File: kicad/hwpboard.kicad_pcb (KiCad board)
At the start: 2 copper layers, 100 x 80 mm, 5 parts, among them J1 Barrel_Jack_Switch, J2 Conn_01x01, J3 Conn_01x01, J4 Conn_01x01, J5 Conn_01x01

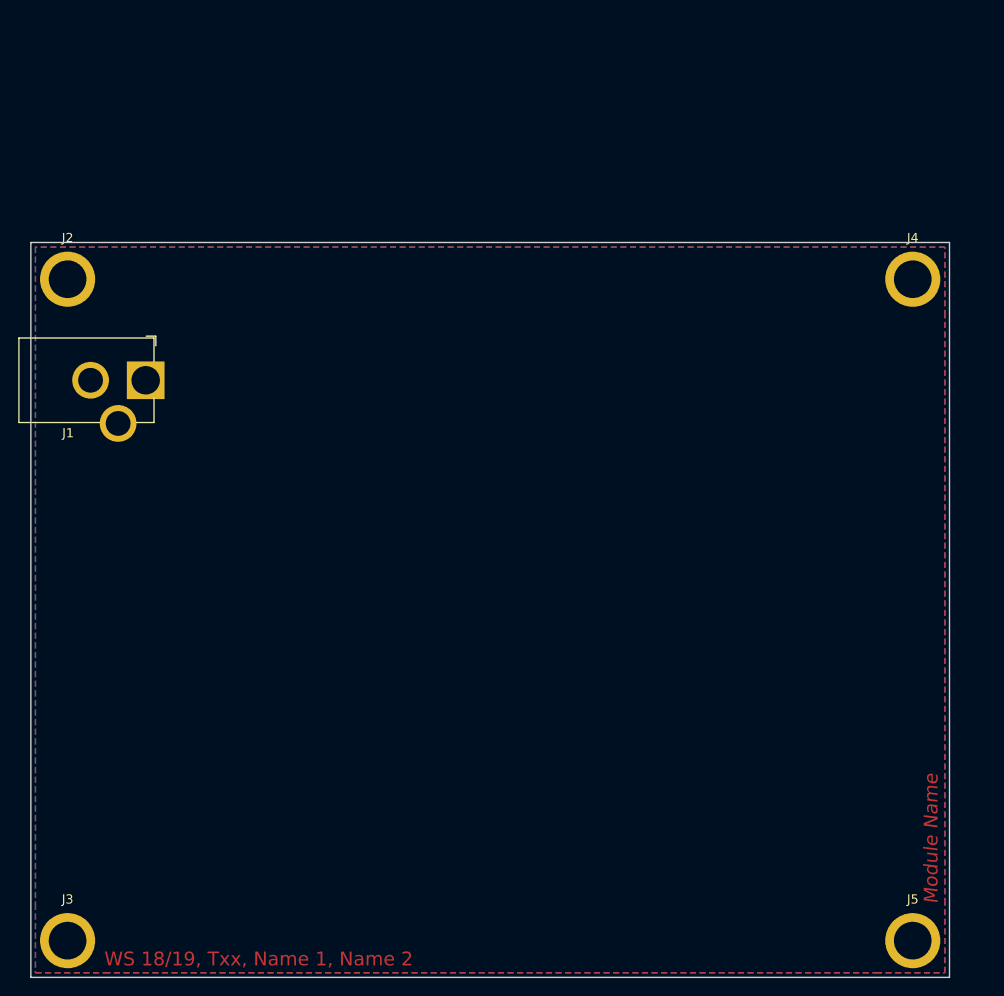
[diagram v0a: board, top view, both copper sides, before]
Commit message: schematic v1.0 ready
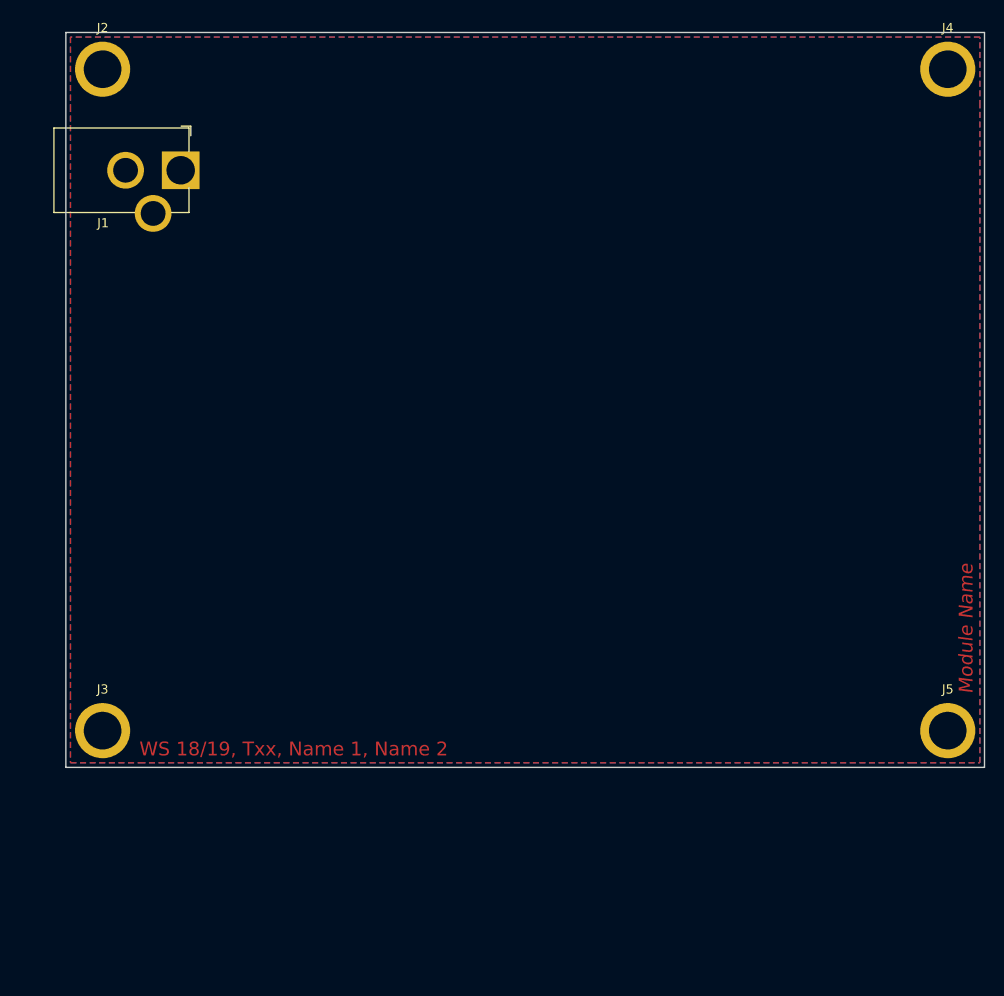
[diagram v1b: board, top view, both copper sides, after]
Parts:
- moved J1 23.2 mm to (121.3, 57.1)
- moved J2 23.2 mm to (112.8, 46.1)
- moved J3 23.2 mm to (112.8, 118.1)
- moved J4 23.2 mm to (204.8, 46.1)
- moved J5 23.2 mm to (204.8, 118.1)
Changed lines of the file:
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@@
-(kicad_pcb (version 20171130) (host pcbnew 5.0.0+dfsg1-2~bpo9+1)
+(kicad_pcb (version 20171130) (host pcbnew 5.0.0-fee4fd1~66~ubuntu18.04.1)
   (general
     (thickness 1.6)
@@
   )
   (module HWP:BarrelJack_Horizontal_CustomHWP (layer F.Cu)
-    (at 117.5 80)
+    (at 121.31 57.14)
     (descr "DC Barrel Jack")
     (tags "Power Jack")
@@
   )
   (module HWP:MountingHole_4.1mm_M4_ISO14580_Pad (layer F.Cu)
-    (at 109 69)
+    (at 112.81 46.14)
     (descr "Mounting Hole 4.3mm, M4, ISO14580")
     (tags "mounting hole 4.3mm m4 iso14580")
@@
   )
   (module HWP:MountingHole_4.1mm_M4_ISO14580_Pad (layer F.Cu)
-    (at 109 141)
+    (at 112.81 118.14)
     (descr "Mounting Hole 4.3mm, M4, ISO14580")
     (tags "mounting hole 4.3mm m4 iso14580")
@@
   )
   (module HWP:MountingHole_4.1mm_M4_ISO14580_Pad (layer F.Cu)
-    (at 201 69)
+    (at 204.81 46.14)
     (descr "Mounting Hole 4.3mm, M4, ISO14580")
     (tags "mounting hole 4.3mm m4 iso14580")
@@
   )
   (module HWP:MountingHole_4.1mm_M4_ISO14580_Pad (layer F.Cu)
-    (at 201 141)
+    (at 204.81 118.14)
     (descr "Mounting Hole 4.3mm, M4, ISO14580")
     (tags "mounting hole 4.3mm m4 iso14580")
@@
   )
   (dimension 80 (width 0.3) (layer Dwgs.User)
-    (gr_text "80 mm" (at 92.900001 105 270) (layer Dwgs.User)
+    (gr_text "80 mm" (at 118.300001 98.65 270) (layer Dwgs.User)
       (effects (font (size 1.5 1.5) (thickness 0.3)))
     )
-    (feature1 (pts (xy 100 145) (xy 94.41358 145)))
-    (feature2 (pts (xy 100 65) (xy 94.41358 65)))
-    (crossbar (pts (xy 95.000001 65) (xy 95.000001 145)))
-    (arrow1a (pts (xy 95.000001 145) (xy 94.41358 143.873496)))
-    (arrow1b (pts (xy 95.000001 145) (xy 95.586422 143.873496)))
-    (arrow2a (pts (xy 95.000001 65) (xy 94.41358 66.126504)))
-    (arrow2b (pts (xy 95.000001 65) (xy 95.586422 66.126504)))
-  )
-  (gr_text "Module Name" (at 203 137 90) (layer F.Cu)
+    (feature1 (pts (xy 125.4 138.65) (xy 119.81358 138.65)))
+    (feature2 (pts (xy 125.4 58.65) (xy 119.81358 58.65)))
+    (crossbar (pts (xy 120.400001 58.65) (xy 120.400001 138.65)))
+    (arrow1a (pts (xy 120.400001 138.65) (xy 119.81358 137.523496)))
+    (arrow1b (pts (xy 120.400001 138.65) (xy 120.986422 137.523496)))
+    (arrow2a (pts (xy 120.400001 58.65) (xy 119.81358 59.776504)))
+    (arrow2b (pts (xy 120.400001 58.65) (xy 120.986422 59.776504)))
+  )
+  (gr_text "Module Name" (at 206.81 114.14 90) (layer F.Cu)
     (effects (font (size 1.5 1.5) (thickness 0.2) italic) (justify left))
   )
-  (gr_text "WS 18/19, Txx, Name 1, Name 2" (at 113 143) (layer F.Cu)
+  (gr_text "WS 18/19, Txx, Name 1, Name 2" (at 116.81 120.14) (layer F.Cu)
     (effects (font (size 1.5 1.5) (thickness 0.2)) (justify left))
   )
   (dimension 100 (width 0.3) (layer Dwgs.User)
-    (gr_text "100 mm" (at 155 52.9) (layer Dwgs.User)
+    (gr_text "100 mm" (at 158.81 30.04) (layer Dwgs.User)
       (effects (font (size 1.5 1.5) (thickness 0.3)))
     )
-    (feature1 (pts (xy 205 60) (xy 205 54.413579)))
-    (feature2 (pts (xy 105 60) (xy 105 54.413579)))
-    (crossbar (pts (xy 105 55) (xy 205 55)))
-    (arrow1a (pts (xy 205 55) (xy 203.873496 55.586421)))
-    (arrow1b (pts (xy 205 55) (xy 203.873496 54.413579)))
-    (arrow2a (pts (xy 105 55) (xy 106.126504 55.586421)))
-    (arrow2b (pts (xy 105 55) (xy 106.126504 54.413579)))
-  )
-  (gr_line (start 105 145) (end 105 65) (layer Edge.Cuts) (width 0.15))
-  (gr_line (start 205 145) (end 105 145) (layer Edge.Cuts) (width 0.15))
-  (gr_line (start 205 65) (end 205 145) (layer Edge.Cuts) (width 0.15))
-  (gr_line (start 105 65) (end 205 65) (layer Edge.Cuts) (width 0.15))
+    (feature1 (pts (xy 208.81 37.14) (xy 208.81 31.553579)))
+    (feature2 (pts (xy 108.81 37.14) (xy 108.81 31.553579)))
+    (crossbar (pts (xy 108.81 32.14) (xy 208.81 32.14)))
+    (arrow1a (pts (xy 208.81 32.14) (xy 207.683496 32.726421)))
+    (arrow1b (pts (xy 208.81 32.14) (xy 207.683496 31.553579)))
+    (arrow2a (pts (xy 108.81 32.14) (xy 109.936504 32.726421)))
+    (arrow2b (pts (xy 108.81 32.14) (xy 109.936504 31.553579)))
+  )
+  (gr_line (start 108.81 122.14) (end 108.81 42.14) (layer Edge.Cuts) (width 0.15))
+  (gr_line (start 208.81 122.14) (end 108.81 122.14) (layer Edge.Cuts) (width 0.15))
+  (gr_line (start 208.81 42.14) (end 208.81 122.14) (layer Edge.Cuts) (width 0.15))
+  (gr_line (start 108.81 42.14) (end 208.81 42.14) (layer Edge.Cuts) (width 0.15))
   (zone (net 2) (net_name GND) (layer B.Cu) (hatch none 0.508)
     (connect_pads (clearance 0.508))
@@
     (polygon
       (pts
-        (xy 113 65.5) (xy 105.5 65.5) (xy 105.5 73) (xy 105.5 137) (xy 105.5 144.5)
-        (xy 113 144.5) (xy 197 144.5) (xy 204.5 144.5) (xy 204.5 137) (xy 204.5 73)
-        (xy 204.5 65.5) (xy 197 65.5)
+        (xy 116.81 42.64) (xy 109.31 42.64) (xy 109.31 50.14) (xy 109.31 114.14) (xy 109.31 121.64)
+        (xy 116.81 121.64) (xy 200.81 121.64) (xy 208.31 121.64) (xy 208.31 114.14) (xy 208.31 50.14)
+        (xy 208.31 42.64) (xy 200.81 42.64)
       )
     )
@@
     (polygon
       (pts
-        (xy 113 65.5) (xy 105.5 65.5) (xy 105.5 73) (xy 105.5 137) (xy 105.5 144.5)
-        (xy 113 144.5) (xy 197 144.5) (xy 204.5 144.5) (xy 204.5 137) (xy 204.5 73)
-        (xy 204.5 65.5) (xy 197 65.5)
+        (xy 116.81 42.64) (xy 109.31 42.64) (xy 109.31 50.14) (xy 109.31 114.14) (xy 109.31 121.64)
+        (xy 116.81 121.64) (xy 200.81 121.64) (xy 208.31 121.64) (xy 208.31 114.14) (xy 208.31 50.14)
+        (xy 208.31 42.64) (xy 200.81 42.64)
       )
     )
